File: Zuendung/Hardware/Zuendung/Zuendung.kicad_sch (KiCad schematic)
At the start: 59 parts, among them J1 Conn_01x04, J1 USB_B_Micro, J3 SWD, J5 Conn_01x03, Q1 DMN6140L, Q2 DMN6140L, Q3 MSC090SMA070B, U2 AP2204RA-3.3, U2 USBLC6-2SC6, U5 OPA990, U6 OPA990, U9 STM32G431K8Tx

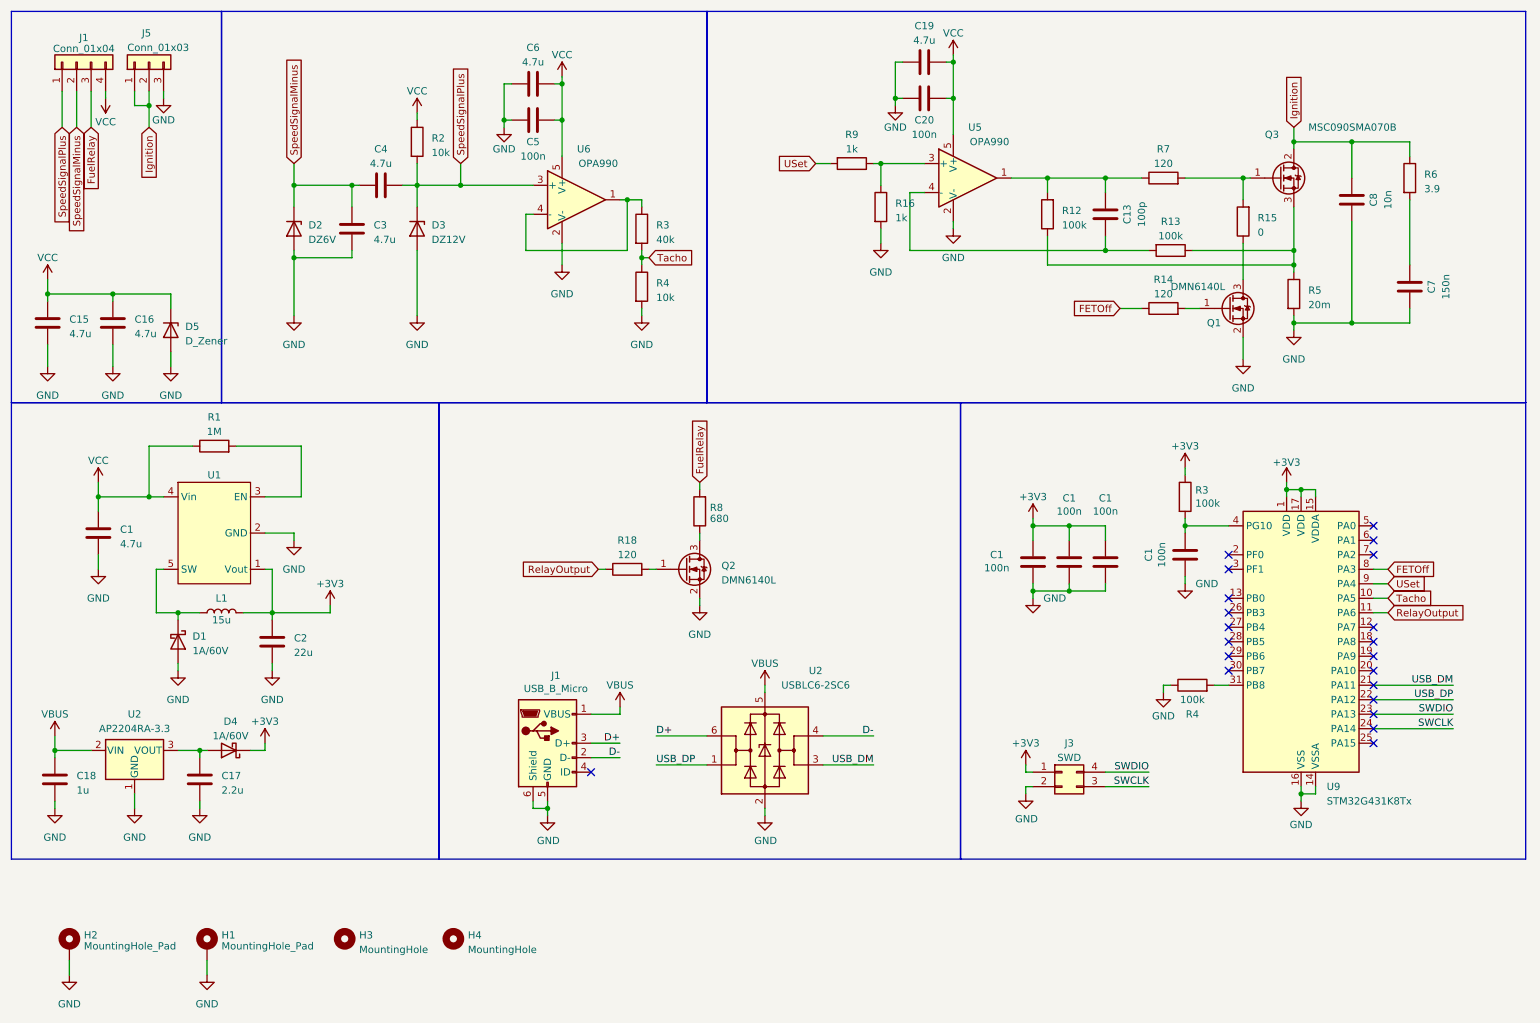
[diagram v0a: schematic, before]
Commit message: changes for Version 2.0
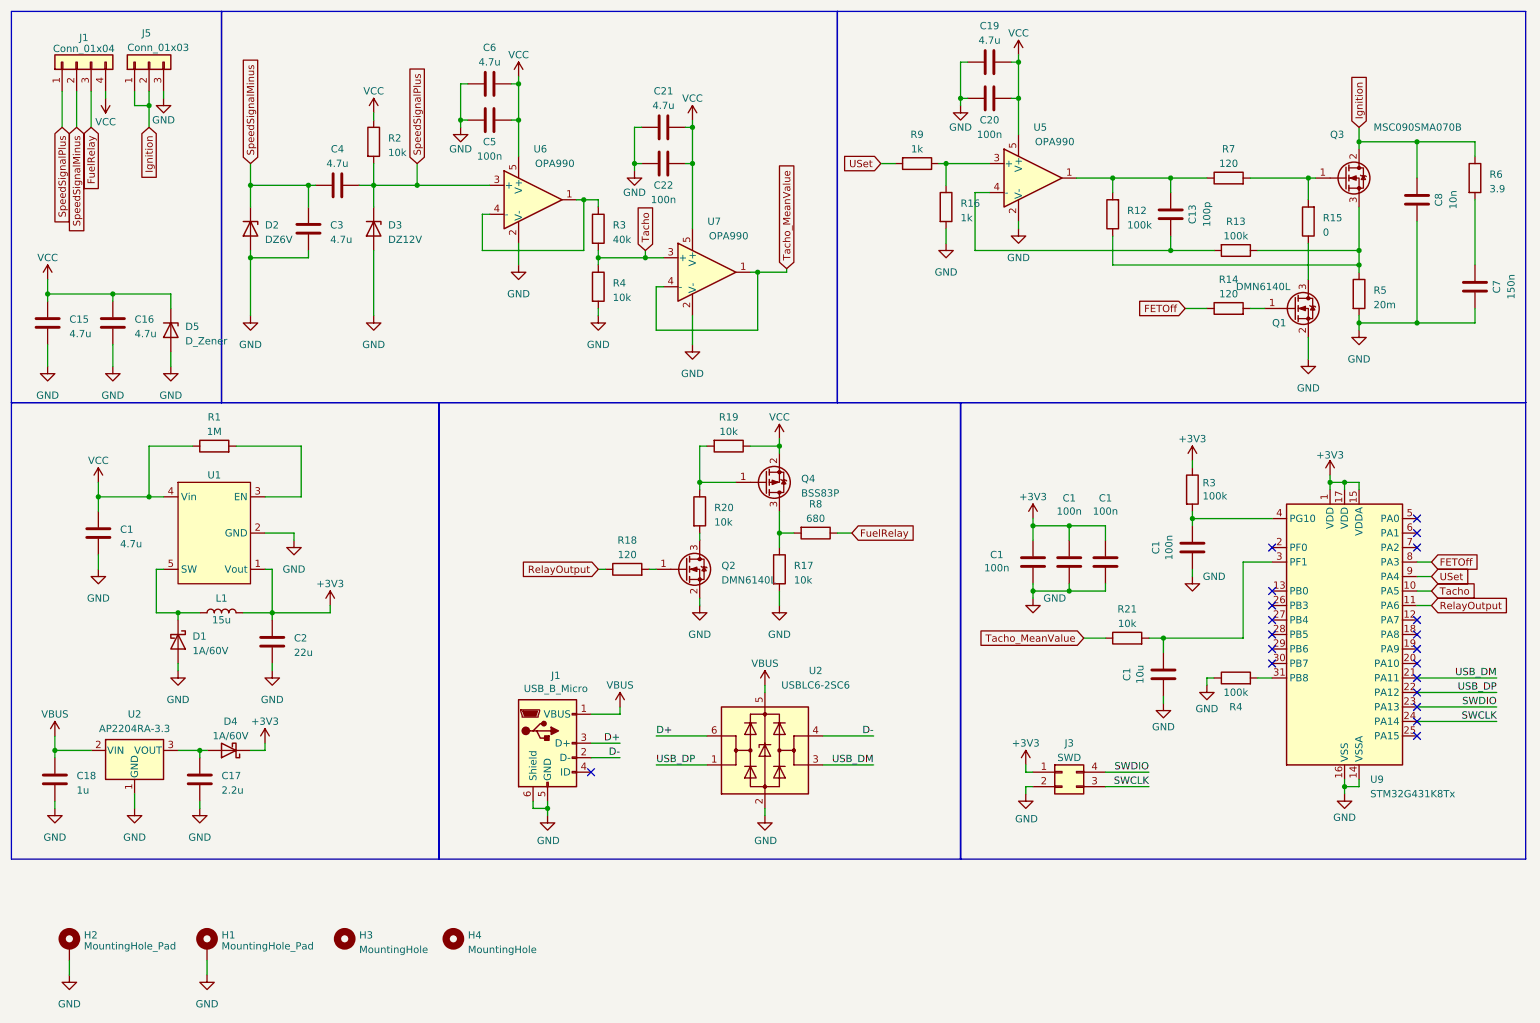
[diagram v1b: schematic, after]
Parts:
- added C1: 10u, Capacitor_SMD:C_0603_1608Metric, symbol Device:C
- added C21: 4.7u, Capacitor_SMD:C_0805_2012Metric, symbol Device:C
- added C22: 100n, Capacitor_SMD:C_0603_1608Metric, symbol Device:C
- added Q4: BSS83P, Package_TO_SOT_SMD:SOT-23, symbol Transistor_FET:BSS83P
- added R17, R19, R20, R21: 10k, Resistor_SMD:R_0603_1608Metric, symbol Device:R
- added U7: OPA990, Package_TO_SOT_SMD:SOT-23-5, symbol Amplifier_Operational:ADA4610-1xRJ
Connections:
- net FuelRelay: now also R8.1; no longer R8.2
- net GND: now also C1.1, C21.2, C22.2, R17.2, U7.2 (V-)
- net Tacho: now also U7.3 (+)
- net VCC: now also C21.1, C22.1, Q4.2 (S), R19.1, U7.5 (V+)
- net at Q2.3 (D): now also R20.2; no longer R8.1
- net at U9.3 (PF1): now also C1.2, R21.2
- new net: Q4.1 (G), R19.2, R20.1
- new net: Q4.3 (D), R17.1, R8.2
- new net Tacho_MeanValue: R21.1, U7.1, U7.4 (-)
- no-connect marks 21 -> 20
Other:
- moved on the sheet: C1, C13, C19, C20, C3, C4, C5, C6, C7, C8, D2, D3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
